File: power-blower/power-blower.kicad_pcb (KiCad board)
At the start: 2 copper layers, 15.8 x 19 mm, 2 parts, among them J1 USB_A, J2 USB_A

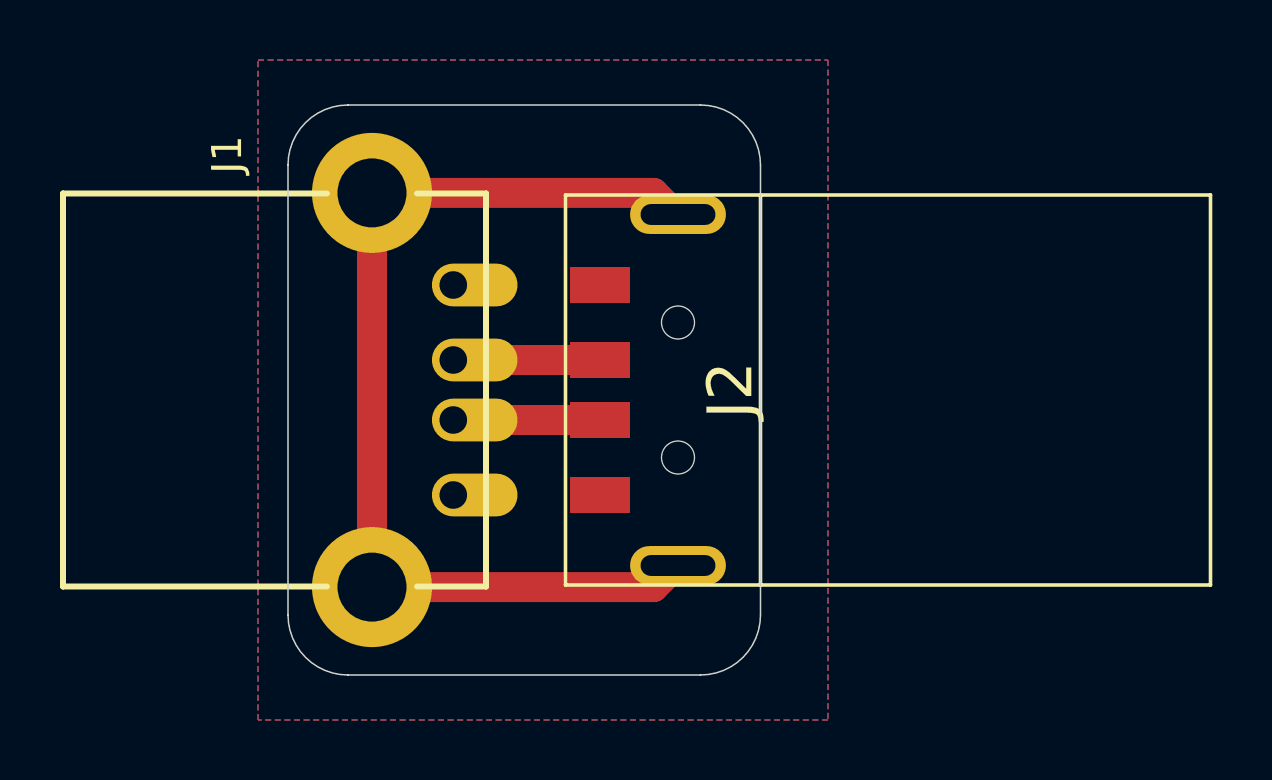
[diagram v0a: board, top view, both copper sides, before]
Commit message: power-blower: as committed
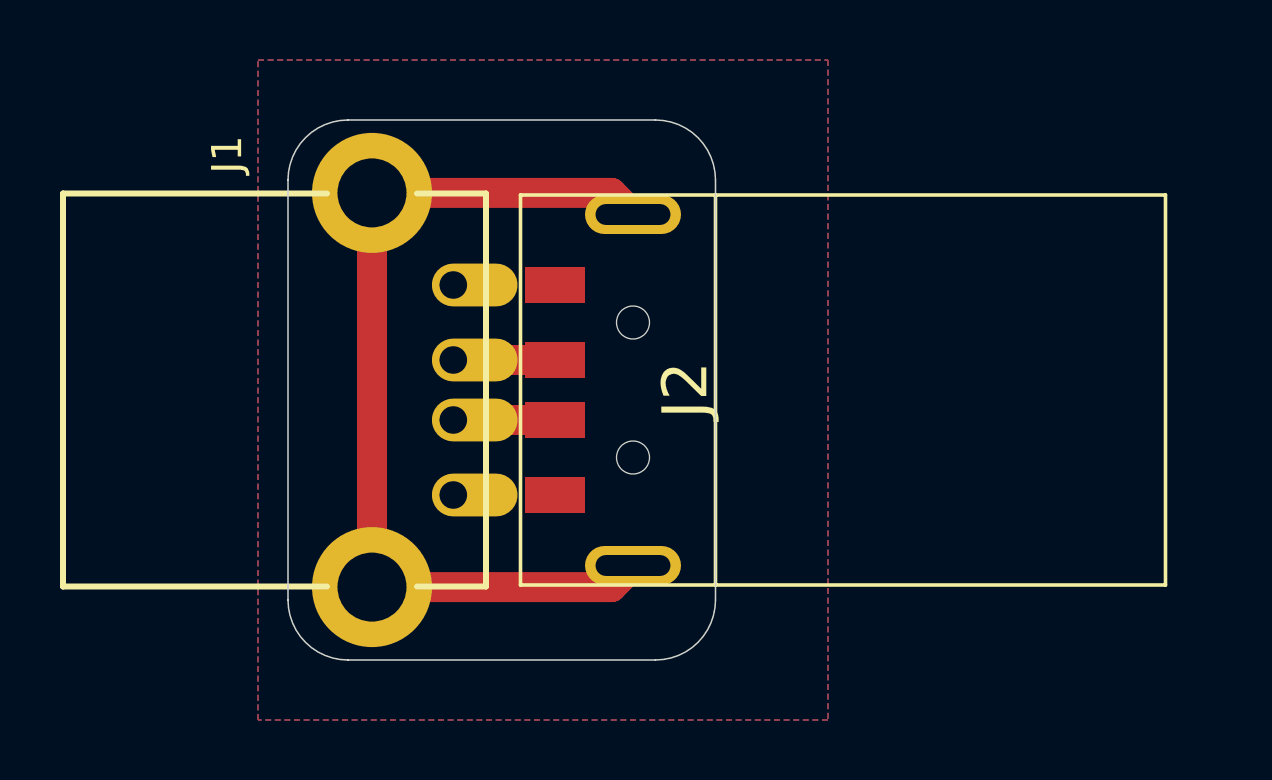
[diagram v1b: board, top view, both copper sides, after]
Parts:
- moved J2 1.50 mm to (167.5, 96.0)
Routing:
- net Net-(J1-Pad5): track 34.2 -> 31.1 mm
- net Net-(J1-Pad3): track 4.89 -> 3.39 mm
- net Net-(J1-Pad2): track 4.89 -> 3.39 mm
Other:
- board size 15.8 x 19 mm -> 14.2 x 18 mm
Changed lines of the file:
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@@
   )
   (module tom-connectors:USB_A_PLUG_MOLEX_480372200 (layer F.Cu)
-    (at 169 96 90)
+    (at 167.5 96 90)
     (descr "Universal Serial Bus (USB) Shielded I/O Plug, Type A, Right-Angle, Surface Mount")
     (attr smd)
@@
       (effects (font (size 1.5 1.5) (thickness 0.2)))
     )
+    (fp_line (start 6.5 17.75) (end -6.5 17.75) (layer F.SilkS) (width 0.12))
+    (fp_line (start 6.5 -3.75) (end 6.5 17.75) (layer F.SilkS) (width 0.12))
+    (fp_line (start -6.5 -3.75) (end 6.5 -3.75) (layer F.SilkS) (width 0.12))
+    (fp_line (start -6.5 -3.75) (end -6.5 17.75) (layer F.SilkS) (width 0.12))
+    (fp_line (start -6.5 -3.75) (end 6.5 -3.75) (layer F.CrtYd) (width 0.12))
+    (fp_line (start 6.5 -3.75) (end 6.5 2.75) (layer F.CrtYd) (width 0.12))
+    (fp_line (start 6.5 2.75) (end -6.5 2.75) (layer F.CrtYd) (width 0.12))
+    (fp_line (start -6.5 2.75) (end -6.5 -3.75) (layer F.CrtYd) (width 0.12))
     (fp_line (start -6.5 2.75) (end 6.5 2.75) (layer F.SilkS) (width 0.12))
-    (fp_line (start -6.5 2.75) (end -6.5 -3.75) (layer F.CrtYd) (width 0.12))
-    (fp_line (start 6.5 2.75) (end -6.5 2.75) (layer F.CrtYd) (width 0.12))
-    (fp_line (start 6.5 -3.75) (end 6.5 2.75) (layer F.CrtYd) (width 0.12))
-    (fp_line (start -6.5 -3.75) (end 6.5 -3.75) (layer F.CrtYd) (width 0.12))
-    (fp_line (start -6.5 -3.75) (end -6.5 17.75) (layer F.SilkS) (width 0.12))
-    (fp_line (start -6.5 -3.75) (end 6.5 -3.75) (layer F.SilkS) (width 0.12))
-    (fp_line (start 6.5 -3.75) (end 6.5 17.75) (layer F.SilkS) (width 0.12))
-    (fp_line (start 6.5 17.75) (end -6.5 17.75) (layer F.SilkS) (width 0.12))
     (pad "" np_thru_hole circle (at 2.25 0 90) (size 1.1 1.1) (drill 1.1) (layers *.Cu *.Mask))
     (pad "" np_thru_hole circle (at -2.25 0 90) (size 1.1 1.1) (drill 1.1) (layers *.Cu *.Mask))
@@
       (effects (font (size 1.001984 1.001984) (thickness 0.015)))
     )
+    (fp_line (start -6.8 -5.1) (end -6.8 -7.85) (layer F.CrtYd) (width 0.05))
+    (fp_line (start -7.8 -5.1) (end -6.8 -5.1) (layer F.CrtYd) (width 0.05))
+    (fp_line (start -7.8 -2.55) (end -7.8 -5.1) (layer F.CrtYd) (width 0.05))
+    (fp_line (start -6.8 -2.55) (end -7.8 -2.55) (layer F.CrtYd) (width 0.05))
+    (fp_line (start -6.8 6.75) (end -6.8 -2.55) (layer F.CrtYd) (width 0.05))
+    (fp_line (start 6.8 6.75) (end -6.8 6.75) (layer F.CrtYd) (width 0.05))
+    (fp_line (start 6.8 -2.55) (end 6.8 6.75) (layer F.CrtYd) (width 0.05))
+    (fp_line (start 7.8 -2.55) (end 6.8 -2.55) (layer F.CrtYd) (width 0.05))
+    (fp_line (start 7.8 -5.1) (end 7.8 -2.55) (layer F.CrtYd) (width 0.05))
+    (fp_line (start 6.8 -5.1) (end 7.8 -5.1) (layer F.CrtYd) (width 0.05))
+    (fp_line (start 6.8 -7.85) (end 6.8 -5.1) (layer F.CrtYd) (width 0.05))
+    (fp_line (start -6.8 -7.85) (end 6.8 -7.85) (layer F.CrtYd) (width 0.05))
+    (fp_line (start 6.55 -7.6) (end 6.55 -5.3) (layer F.SilkS) (width 0.2))
+    (fp_line (start -6.55 -7.6) (end 6.55 -7.6) (layer F.SilkS) (width 0.2))
+    (fp_line (start -6.55 -5.3) (end -6.55 -7.6) (layer F.SilkS) (width 0.2))
+    (fp_line (start 6.55 6.5) (end 6.55 -2.3) (layer F.SilkS) (width 0.2))
+    (fp_line (start -6.55 6.5) (end 6.55 6.5) (layer F.SilkS) (width 0.2))
     (fp_line (start -6.55 -2.3) (end -6.55 6.5) (layer F.SilkS) (width 0.2))
-    (fp_line (start -6.55 6.5) (end 6.55 6.5) (layer F.SilkS) (width 0.2))
-    (fp_line (start 6.55 6.5) (end 6.55 -2.3) (layer F.SilkS) (width 0.2))
-    (fp_line (start -6.55 -5.3) (end -6.55 -7.6) (layer F.SilkS) (width 0.2))
-    (fp_line (start -6.55 -7.6) (end 6.55 -7.6) (layer F.SilkS) (width 0.2))
-    (fp_line (start 6.55 -7.6) (end 6.55 -5.3) (layer F.SilkS) (width 0.2))
-    (fp_line (start -6.8 -7.85) (end 6.8 -7.85) (layer F.CrtYd) (width 0.05))
-    (fp_line (start 6.8 -7.85) (end 6.8 -5.1) (layer F.CrtYd) (width 0.05))
-    (fp_line (start 6.8 -5.1) (end 7.8 -5.1) (layer F.CrtYd) (width 0.05))
-    (fp_line (start 7.8 -5.1) (end 7.8 -2.55) (layer F.CrtYd) (width 0.05))
-    (fp_line (start 7.8 -2.55) (end 6.8 -2.55) (layer F.CrtYd) (width 0.05))
-    (fp_line (start 6.8 -2.55) (end 6.8 6.75) (layer F.CrtYd) (width 0.05))
-    (fp_line (start 6.8 6.75) (end -6.8 6.75) (layer F.CrtYd) (width 0.05))
-    (fp_line (start -6.8 6.75) (end -6.8 -2.55) (layer F.CrtYd) (width 0.05))
-    (fp_line (start -6.8 -2.55) (end -7.8 -2.55) (layer F.CrtYd) (width 0.05))
-    (fp_line (start -7.8 -2.55) (end -7.8 -5.1) (layer F.CrtYd) (width 0.05))
-    (fp_line (start -7.8 -5.1) (end -6.8 -5.1) (layer F.CrtYd) (width 0.05))
-    (fp_line (start -6.8 -5.1) (end -6.8 -7.85) (layer F.CrtYd) (width 0.05))
     (pad 4 thru_hole oval (at 3.5 -6.51 270) (size 1.428 2.856) (drill oval 0.92 (offset 0 -0.714)) (layers *.Cu *.Mask)
       (net 6 GND))
@@
     (effects (font (size 1.5 1.5) (thickness 0.25)) (justify mirror))
   )
-  (gr_arc (start 169.75 103.5) (end 169.75 105.5) (angle -90) (layer Edge.Cuts) (width 0.05))
-  (gr_line (start 158 105.5) (end 169.75 105.5) (layer Edge.Cuts) (width 0.05))
-  (gr_line (start 156 88.5) (end 156 103.5) (layer Edge.Cuts) (width 0.05))
-  (gr_arc (start 158 103.5) (end 156 103.5) (angle -90) (layer Edge.Cuts) (width 0.05))
-  (gr_line (start 169.75 86.5) (end 158 86.5) (layer Edge.Cuts) (width 0.05))
-  (gr_arc (start 169.75 88.5) (end 171.75 88.5) (angle -90) (layer Edge.Cuts) (width 0.05))
-  (gr_arc (start 158 88.5) (end 158 86.5) (angle -90) (layer Edge.Cuts) (width 0.05))
-  (gr_line (start 171.75 103.5) (end 171.75 88.5) (layer Edge.Cuts) (width 0.05))
-  (segment (start 161.51 97) (end 166.4 97) (width 1) (layer F.Cu) (net 1))
-  (segment (start 161.51 95) (end 166.4 95) (width 1) (layer F.Cu) (net 2))
+  (gr_arc (start 168.25 103) (end 168.25 105) (angle -90) (layer Edge.Cuts) (width 0.05))
+  (gr_line (start 158 105) (end 168.25 105) (layer Edge.Cuts) (width 0.05))
+  (gr_line (start 156 89) (end 156 103) (layer Edge.Cuts) (width 0.05))
+  (gr_arc (start 158 103) (end 156 103) (angle -90) (layer Edge.Cuts) (width 0.05))
+  (gr_line (start 168.25 87) (end 158 87) (layer Edge.Cuts) (width 0.05))
+  (gr_arc (start 168.25 89) (end 170.25 89) (angle -90) (layer Edge.Cuts) (width 0.05))
+  (gr_arc (start 158 89) (end 158 87) (angle -90) (layer Edge.Cuts) (width 0.05))
+  (gr_line (start 170.25 103) (end 170.25 89) (layer Edge.Cuts) (width 0.05))
+  (segment (start 164.9 97) (end 161.51 97) (width 1) (layer F.Cu) (net 1))
+  (segment (start 164.9 95) (end 161.51 95) (width 1) (layer F.Cu) (net 2))
   (segment (start 158.8 102.57) (end 158.8 89.43) (width 1) (layer F.Cu) (net 3))
-  (segment (start 168.18 89.43) (end 169 90.25) (width 1) (layer F.Cu) (net 3))
-  (segment (start 158.8 89.43) (end 168.18 89.43) (width 1) (layer F.Cu) (net 3))
-  (segment (start 168.18 102.57) (end 169 101.75) (width 1) (layer F.Cu) (net 3))
-  (segment (start 158.8 102.57) (end 168.18 102.57) (width 1) (layer F.Cu) (net 3))
+  (segment (start 166.78 89.43) (end 167.5 90.15) (width 1) (layer F.Cu) (net 3))
+  (segment (start 158.8 89.43) (end 166.78 89.43) (width 1) (layer F.Cu) (net 3))
+  (segment (start 166.78 102.57) (end 167.5 101.85) (width 1) (layer F.Cu) (net 3))
+  (segment (start 158.8 102.57) (end 166.78 102.57) (width 1) (layer F.Cu) (net 3))
   (zone (net 6) (net_name GND) (layer F.Cu) (hatch edge 0.508)
     (connect_pads (clearance 0.254))
